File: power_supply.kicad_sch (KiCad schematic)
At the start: 19 parts, among them U7 FT230XS

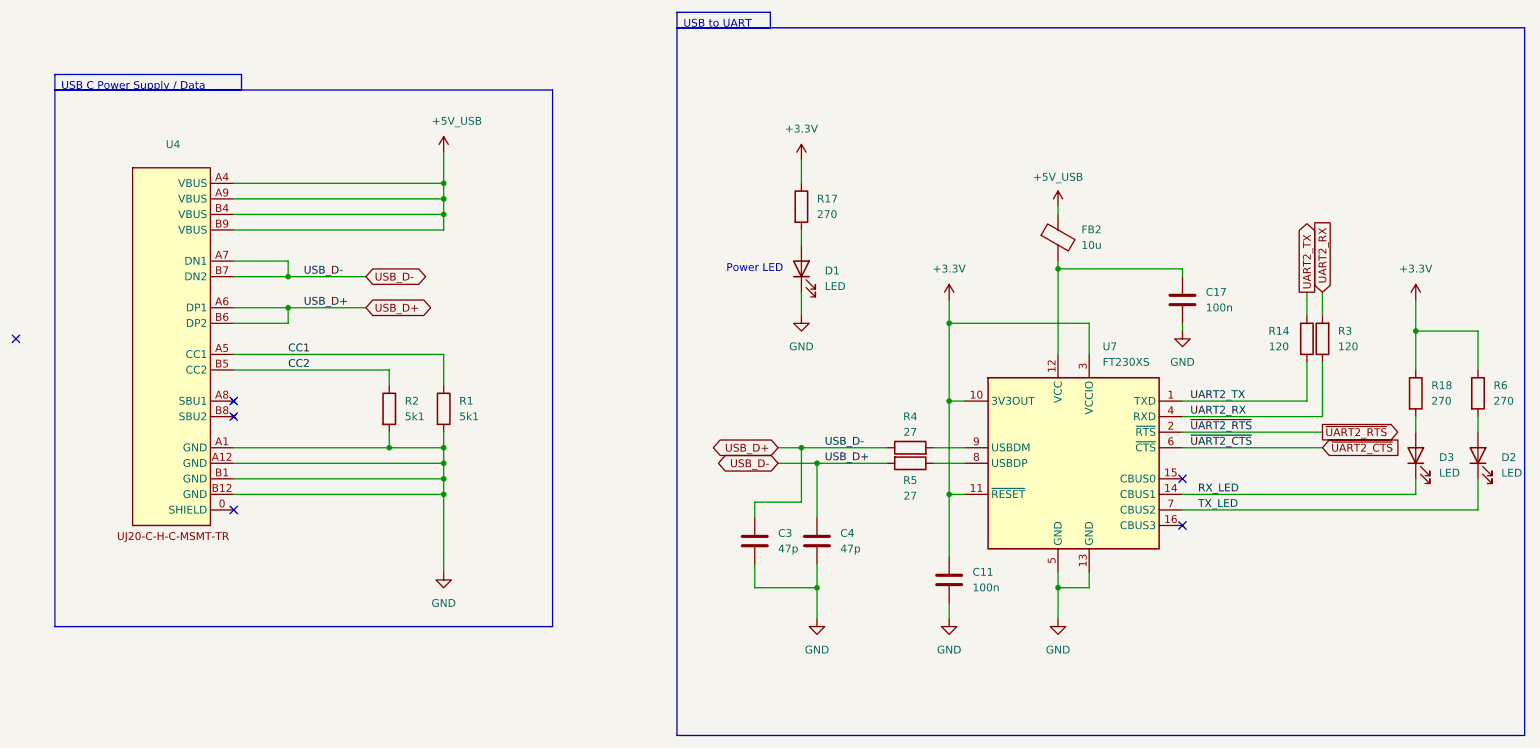
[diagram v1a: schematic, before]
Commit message: fsdfsdf
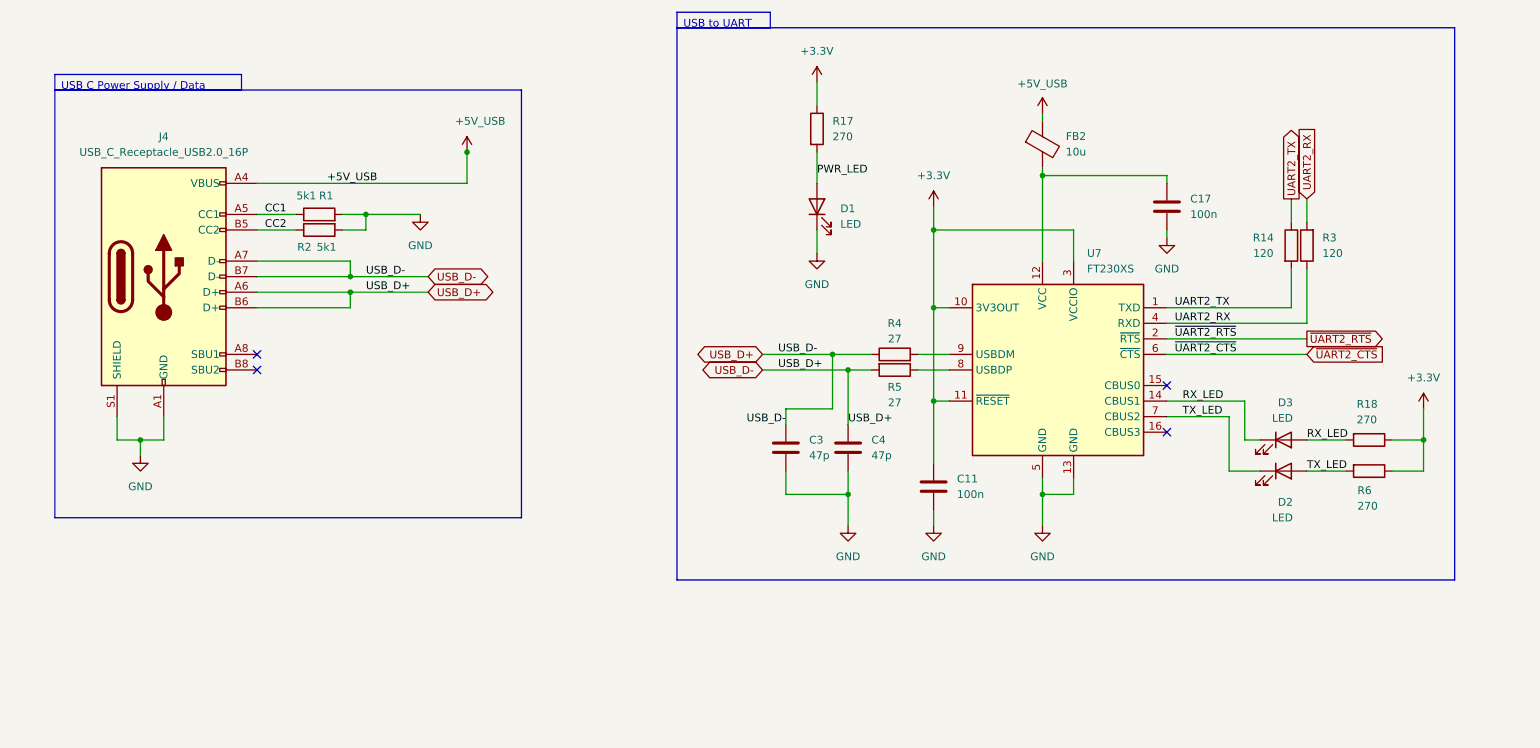
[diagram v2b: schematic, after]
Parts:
- removed U4: ~, custom:640-USB4215-03-A, symbol custom:UJ20-C-H-C-MSMT-TR (USB C 16 Pin)
- added J4: USB_C_Receptacle_USB2.0_16P, custom:640-USB4215-03-A, symbol Connector:USB_C_Receptacle_USB2.0_16P
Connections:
- net +5V_USB: now also J4.A4 (VBUS), J4.A9 (VBUS), J4.B4 (VBUS), J4.B9 (VBUS)
- net CC1: now also J4.A5 (CC1)
- net CC2: now also J4.B5 (CC2)
- net GND: now also J4.A1 (GND), J4.A12 (GND), J4.B1 (GND), J4.B12 (GND), J4.S1 (SHIELD)
- net RX_LED: now also D3.2 (A), R18.2
- net TX_LED: now also D2.2 (A), R6.2
- net USB_D+: now also J4.A6 (D+), J4.A7 (D-), J4.B6 (D+), J4.B7 (D-)
- net PWR_LED: now reaches D1.2 (A), R17.2
- no-connect marks 6 -> 4
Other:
- note removed: "Power LED"
- moved on the sheet: C11, C17, C3, C4, D1, D2, D3, FB2, R1, R14, R17, R18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
